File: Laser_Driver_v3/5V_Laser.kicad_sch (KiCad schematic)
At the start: 19 parts, among them U14 MC7812CTG, U15 MC7808CTG, U16 LT3045EMSE 5V, U17 LT3045EMSE 5V

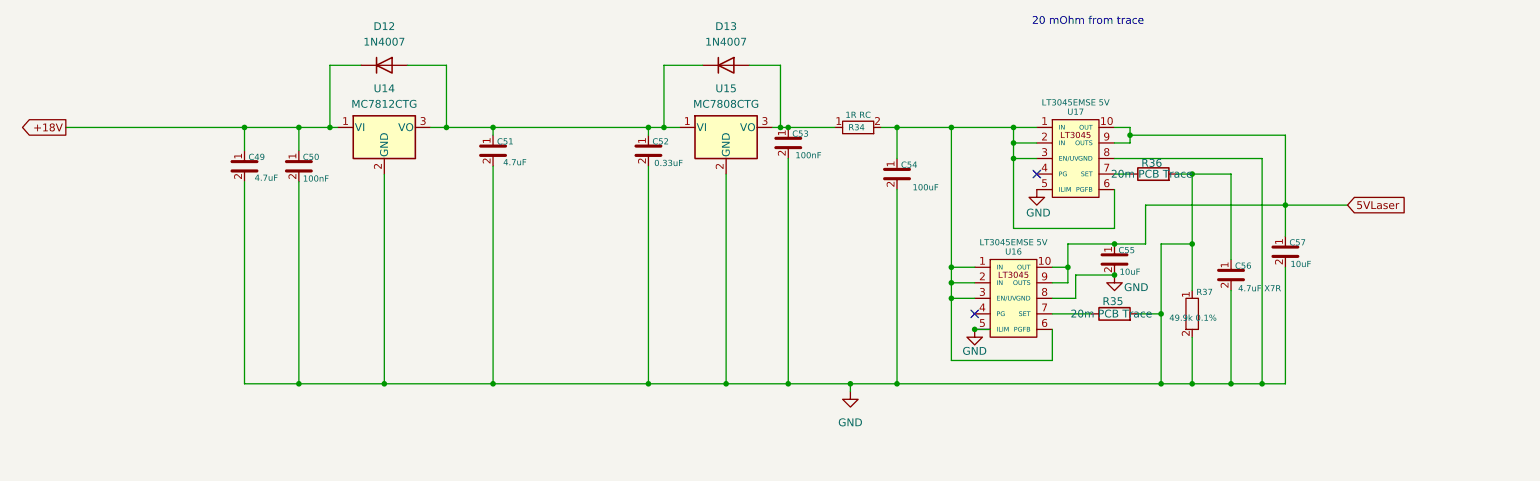
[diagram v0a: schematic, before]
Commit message: Working through power supply layout and footprints
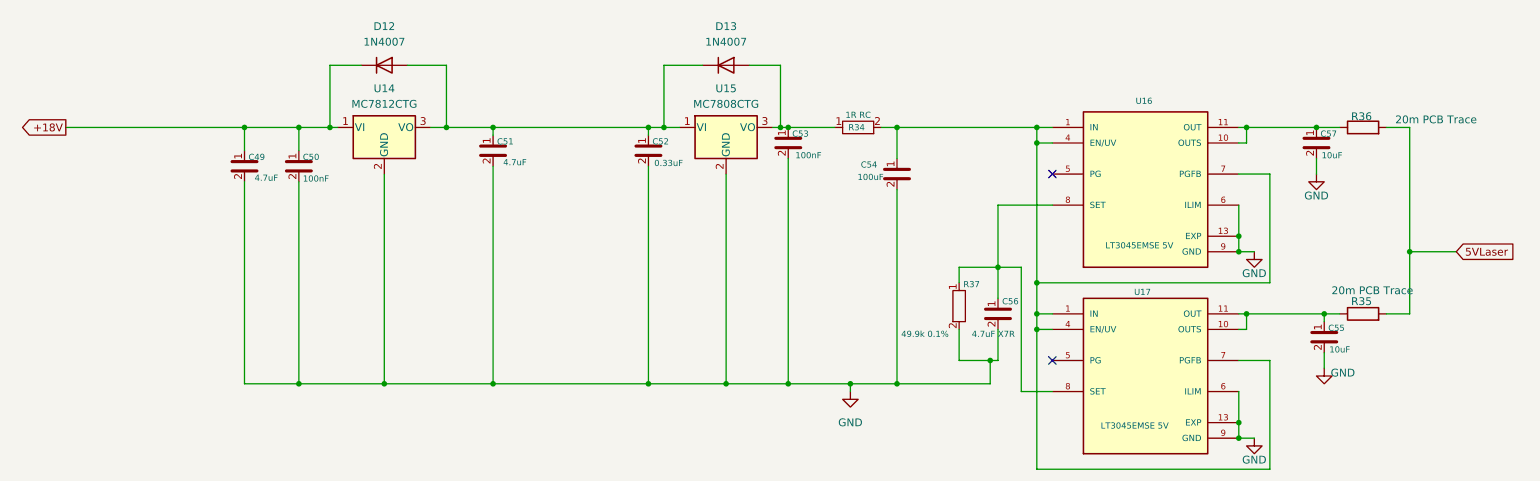
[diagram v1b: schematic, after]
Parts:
- removed U16: LT3045EMSE 5V, Package_SO:Analog_MSOP-12-16-1EP_3x4.039mm_P0.5mm_EP1.651x2.845mm_ThermalVias, symbol Regulator_Linear:LT3042
- added U17: LT3045EMSE 5V, Package_SO:MSOP-12-1EP_3x4.039mm_P0.65mm_EP1.651x2.845mm_ThermalVias, symbol LT3045IMSE_TRPBF:LT3045IMSE_TRPBF
- D12, D13: footprint Diode_THT:D_DO-41_SOD81_P10.16mm_Horizontal -> Diode_THT:D_DO-15_P12.70mm_Horizontal
- U16: renamed from U17; footprint Package_SO:Analog_MSOP-12-16-1EP_3x4.039mm_P0.5mm_EP1.651x2.845mm_ThermalVias -> Package_SO:MSOP-12-1EP_3x4.039mm_P0.65mm_EP1.651x2.845mm_ThermalVias; symbol Regulator_Linear:LT3042 -> LT3045IMSE_TRPBF:LT3045IMSE_TRPBF; Availability (none) -> In Stock; Check_prices (none) -> https://www.snapeda.com/parts/LT3045IMSE%23TRPBF/Analog+Dev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; DUPLICATE (none) -> LT3045HMSE#PBF-,-LT3045EMSE#WPBF-,-LT3045IMSE#WPBF-,-LT3045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; MANUFACTURER (none) -> Analog Devices; MAXIMUM_PACKAGE_HEIGHT (none) -> 1.1mm; MF (none) -> Analog Devices; MP (none) -> LT3045IMSE#TRPBF; PARTREV (none) -> D; Package (none) -> MSOP -12 Analog Devices; Price (none) -> None; Purchase-URL (none) -> https://www.snapeda.com/api/url_track_click_mouser/?unipart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; STANDARD (none) -> IPC-7351B; SnapEDA_Link (none) -> https://www.snapeda.com/parts/LT3045IMSE%23TRPBF/Analog+Dev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
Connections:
- net 5VLaser: now also R35.2, R36.2; no longer C55.1, C57.1, U16.10 (OUT), U16.9 (OUTS)
- net GND: now also U16.13 (EXP), U16.6 (ILIM), U16.9 (GND), U17.13 (EXP), U17.6 (ILIM), U17.9 (GND); no longer C56.1, R35.2, R36.2, R37.1, U16.5 (ILIM), U16.8 (GND)
- net at C54.1, R34.2, U16.1 (IN)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: now also U16.4 (EN/UV), U16.7 (PGFB), U17.1 (IN), U17.2 (IN), U17.3 (IN), U17.4 (EN/UV), U17.7 (PGFB); no longer U16.6 (PGFB)
- net at R35.1: now also C55.1, U17.10 (OUTS), U17.11 (OUT), U17.12 (OUT)
- net at R36.1: now also C57.1, U16.10 (OUTS), U16.11 (OUT), U16.12 (OUT); no longer U16.7 (SET)
- new net: C56.1, R37.1, U16.8 (SET), U17.8 (SET)
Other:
- note removed: "20 mOhm from trace"
- moved on the sheet: C55, C56, C57, R35, R36, R37
